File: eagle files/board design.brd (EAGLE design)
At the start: 115.6 x 89.5 mm, 36 parts, among them IC1 7805T

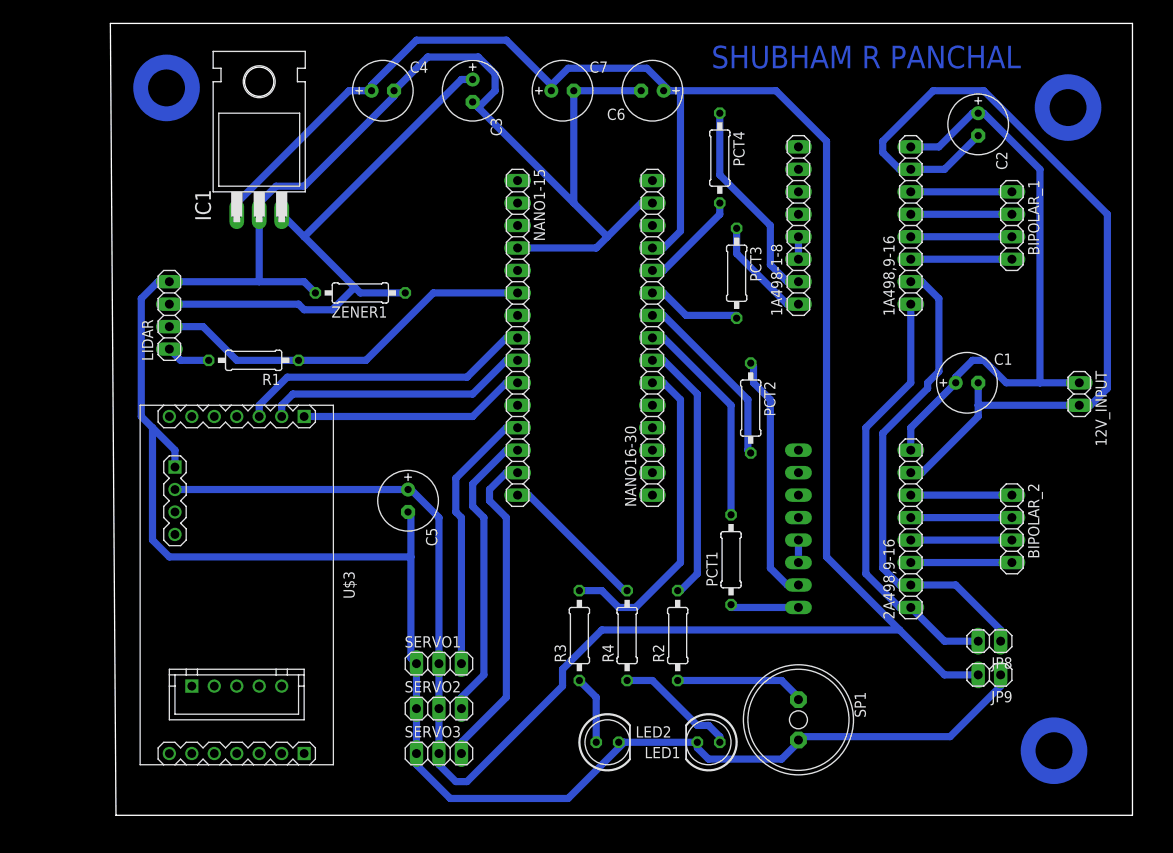
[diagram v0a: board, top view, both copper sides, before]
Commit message: 12/2/19
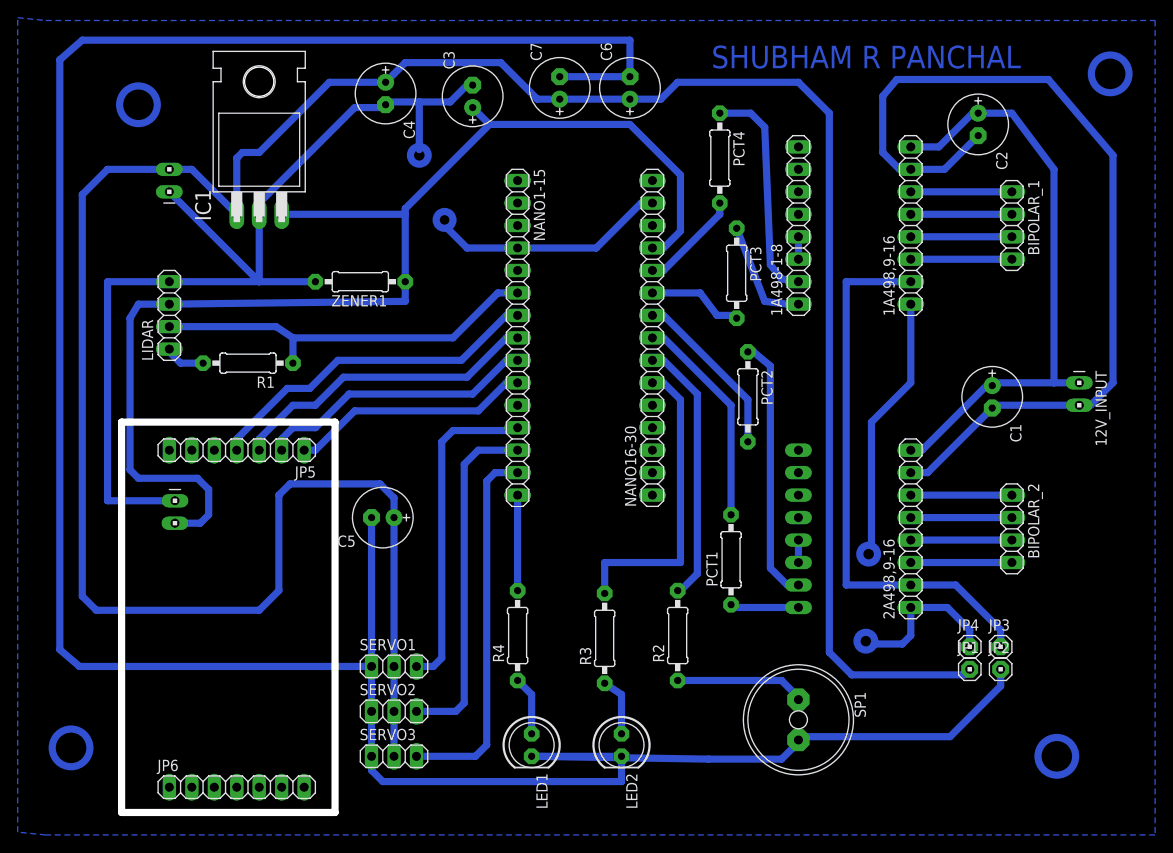
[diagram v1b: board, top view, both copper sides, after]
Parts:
- removed JP8, JP9: (no value), pinhead:1X02
- removed U$3: DRIVER-ULN2003#MC, uln2003:DRIVER-ULN2003#MC
- added 5V_INPUT1, 5V_INPUT2: (no value), pinhead:1X02
- added JP1, JP2, JP3, JP4: (no value), pinhead:1X01
- added JP5, JP6: (no value), pinhead:1X07
- moved LED1 20.0 mm to (47.9, 4.13), turned to 270 degrees
- moved R4 12.4 mm to (46.4, 16.5)
- moved SERVO1 5.09 mm to (32.4, 13.0)
- moved SERVO2 5.09 mm to (32.4, 7.94)
- moved SERVO3 5.09 mm to (32.4, 2.86)
- moved C5 3.43 mm to (31.1, 29.8), turned to 180 degrees
- moved C1 3.27 mm to (100.0, 43.5), turned to 270 degrees
- moved R3 2.88 mm to (56.2, 16.2)
- moved C6 2.56 mm to (59.1, 78.4), turned to 90 degrees
- moved LED2 1.62 mm to (58.1, 4.13), turned to 270 degrees
- moved PCT2 1.31 mm to (72.4, 43.5)
- moved ZENER1 1.27 mm to (28.6, 56.5)
- moved R1 0.71 mm to (15.9, 47.3)
- moved C3 0.64 mm to (41.3, 77.5), turned to 90 degrees
- moved C4 0.45 mm to (31.4, 77.8), turned to 270 degrees
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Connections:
- removed net GND: C3.-, C4.-, C5.-, C6.-, C7.-, IC1.2, JP9.1, LED1.K, LED2.K, LIDAR.4, NANO1-15.4, NANO16-30.14, SERVO1.1, SERVO2.1, SERVO3.1, SP1.+, U$3.J3.1, ZENER1.2
- new net N$36: C5.-, C6.-, C7.-, JP2.1, LED1.K, LED2.K, SERVO1.1, SERVO2.1, SERVO3.1, SP1.+
- new net N$38: 5V_INPUT1.1, 5V_INPUT2.1, C3.-, C4.-, IC1.2, LIDAR.4, NANO1-15.4, NANO16-30.14, ZENER1.2
- net 5V: now also 5V_INPUT1.2, JP1.1; no longer JP9.2, NANO16-30.12, U$3.J3.2
- net GUC: now also JP4.1; no longer JP8.2
- net N$1: now also JP5.4; no longer U$3.J1.4
- net N$2: now also JP5.3; no longer U$3.J1.3
- net N$3: now also JP5.2; no longer U$3.J1.2
- net N$37: now also 5V_INPUT2.2, NANO16-30.12
- net N$4: now also JP5.1; no longer U$3.J1.1
- net VUC: now also JP3.1; no longer JP8.1
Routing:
- net N$36: track 0.00 -> 309.1 mm
- net GND: track 298.0 -> 0.00 mm
- net N$38: track 0.00 -> 140.4 mm
- net N$37: track 66.3 -> 140.9 mm
- net N$1: track 0.00 -> 38.8 mm
- net 5V: track 293.2 -> 304.1 mm
- net VUC: track 54.6 -> 63.1 mm
- net N$17: track 13.7 -> 6.69 mm
- net N$26: track 30.6 -> 36.9 mm
- net N$18: track 16.9 -> 10.8 mm
- net N$22: track 97.1 -> 103.2 mm
- net N$27: track 33.6 -> 39.5 mm
- net N$28: track 36.7 -> 42.2 mm
- net N$33: track 36.7 -> 34.4 mm
- net GUC: track 48.4 -> 46.5 mm
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- added copper zone on layer 16, net N$39
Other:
- board size 115.6 x 89.5 mm -> 24.1 x 44.1 mm
